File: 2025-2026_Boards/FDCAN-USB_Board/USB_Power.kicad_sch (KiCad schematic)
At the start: 8 parts, among them J7 USB4110-GF-A, U1 AMS1117-3.3, U2 USBLC6-2SC6

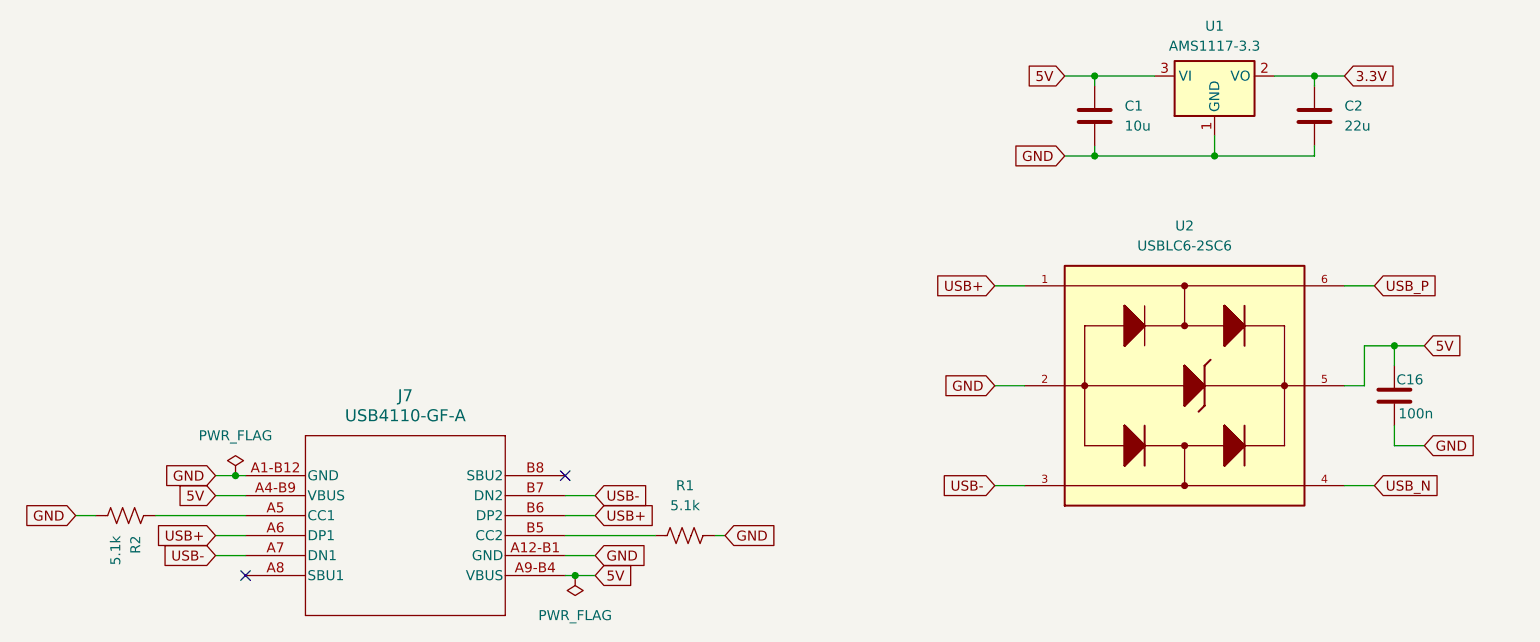
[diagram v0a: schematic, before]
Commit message: Final Design Reupload
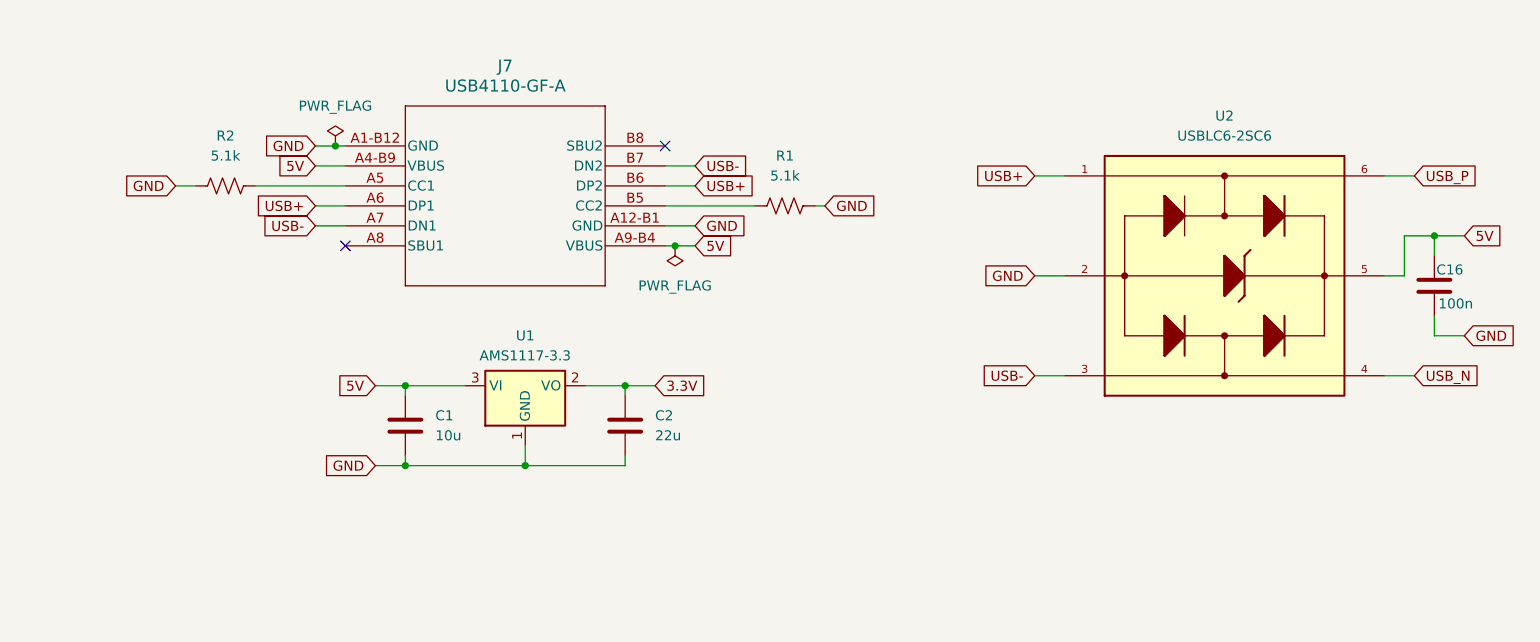
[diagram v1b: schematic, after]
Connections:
- net GND: now also R2.2; no longer R2.1
- net at J7.A5 (CC1): now also R2.1; no longer R2.2
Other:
- moved on the sheet: C1, C16, C2, J7, R1, U1, U2
